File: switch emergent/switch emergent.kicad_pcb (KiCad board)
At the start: 2 copper layers, 38.5 x 58.4 mm, 35 parts, among them J1 Conn_02x04_Odd_Even, J2 Conn_01x06, J3 Conn_01x09, J4 Conn_01x10, J5 Conn_01x10

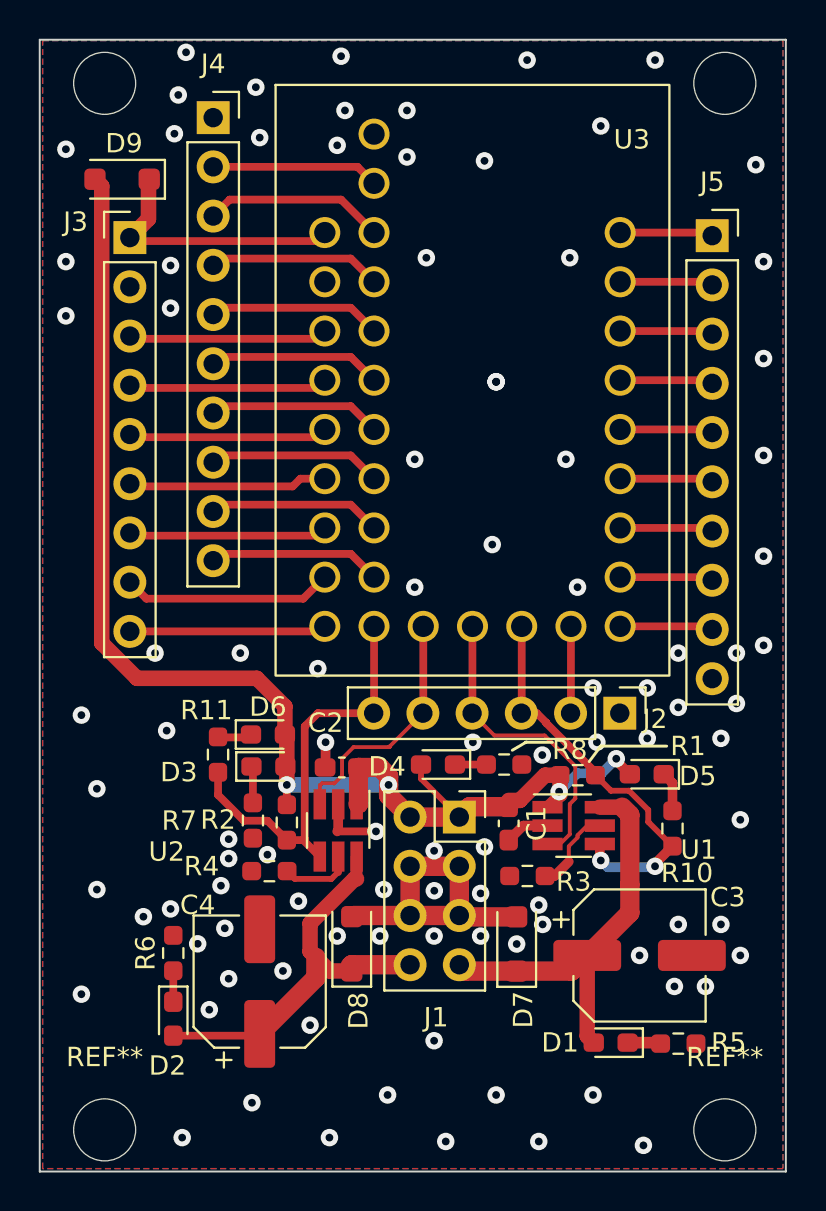
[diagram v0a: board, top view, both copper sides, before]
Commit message: v0.2 Ordered
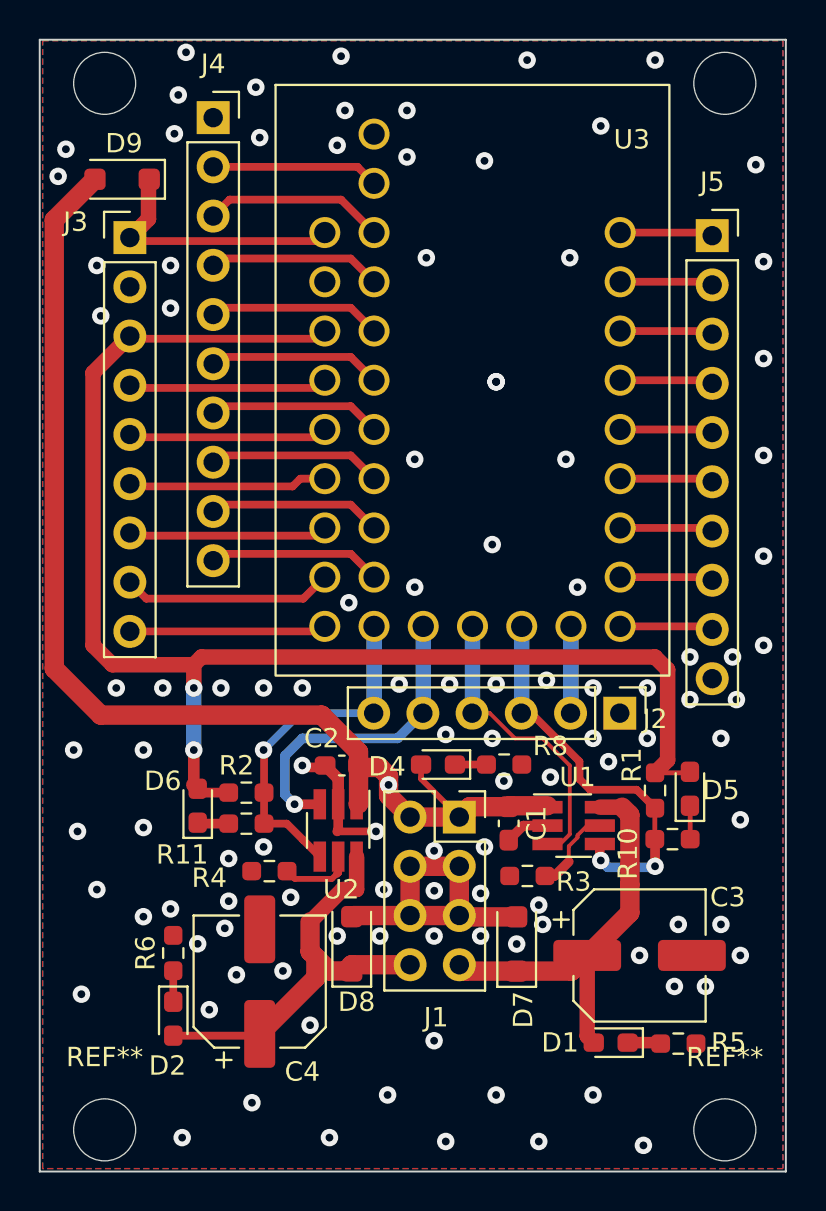
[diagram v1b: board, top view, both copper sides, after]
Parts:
- removed D3: LED, LED_SMD:LED_0603_1608Metric_Pad1.05x0.95mm_HandSolder
- removed R7: 240, Resistor_SMD:R_0603_1608Metric_Pad0.98x0.95mm_HandSolder
- moved D6 5.16 mm to (64.8, 103.3), turned to 90 degrees
- moved R1 4.06 mm to (88.4, 102.5), turned to -90 degrees
- moved R11 3.85 mm to (67.3, 104.2), turned to 0 degrees
- moved R2 2.59 mm to (67.3, 102.6), turned to 0 degrees
- moved D5 2.35 mm to (90.2, 102.4), turned to 90 degrees
- moved R10 0.55 mm to (89.3, 105.0), turned to 180 degrees
- moved C2 0.10 mm to (72.2, 101.2)
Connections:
- D5 pad 2: VBUS -> +3.3V
- D6 pad 2: VBUS -> +3.3V
- J3 pad 3: Net-(J3-Pin_3) -> +3.3V
- R1 pad 1: VBUS -> +3.3V
- R2 pad 1: VBUS -> +3.3V
- U3 pad 30: Net-(J3-Pin_3) -> +3.3V
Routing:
- net +3.3V: track 0.00 -> 73.1 mm, vias 0 -> 2
- net Net-(J3-Pin_3): track 10.3 -> 0.00 mm
- net VBUS: track 70.0 -> 61.5 mm, vias 4 -> 1
- net EN2: track 12.9 -> 16.6 mm, vias 0 -> 1
- net nFLT2: track 22.0 -> 18.4 mm, vias 0 -> 1
- net GND: track 23.1 -> 25.3 mm, vias 97 -> 108
- net Net-(D3-K): track 1.67 -> 0.00 mm
